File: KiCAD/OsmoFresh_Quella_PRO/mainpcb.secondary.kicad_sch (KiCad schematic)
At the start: 92 parts, among them K2 5A 250Vac, Q2 NMOS, Q3 NPN, Q4 PMOS, Q5 NPN, Q6 NPN, Q8 NPN, U4 ULN2003A

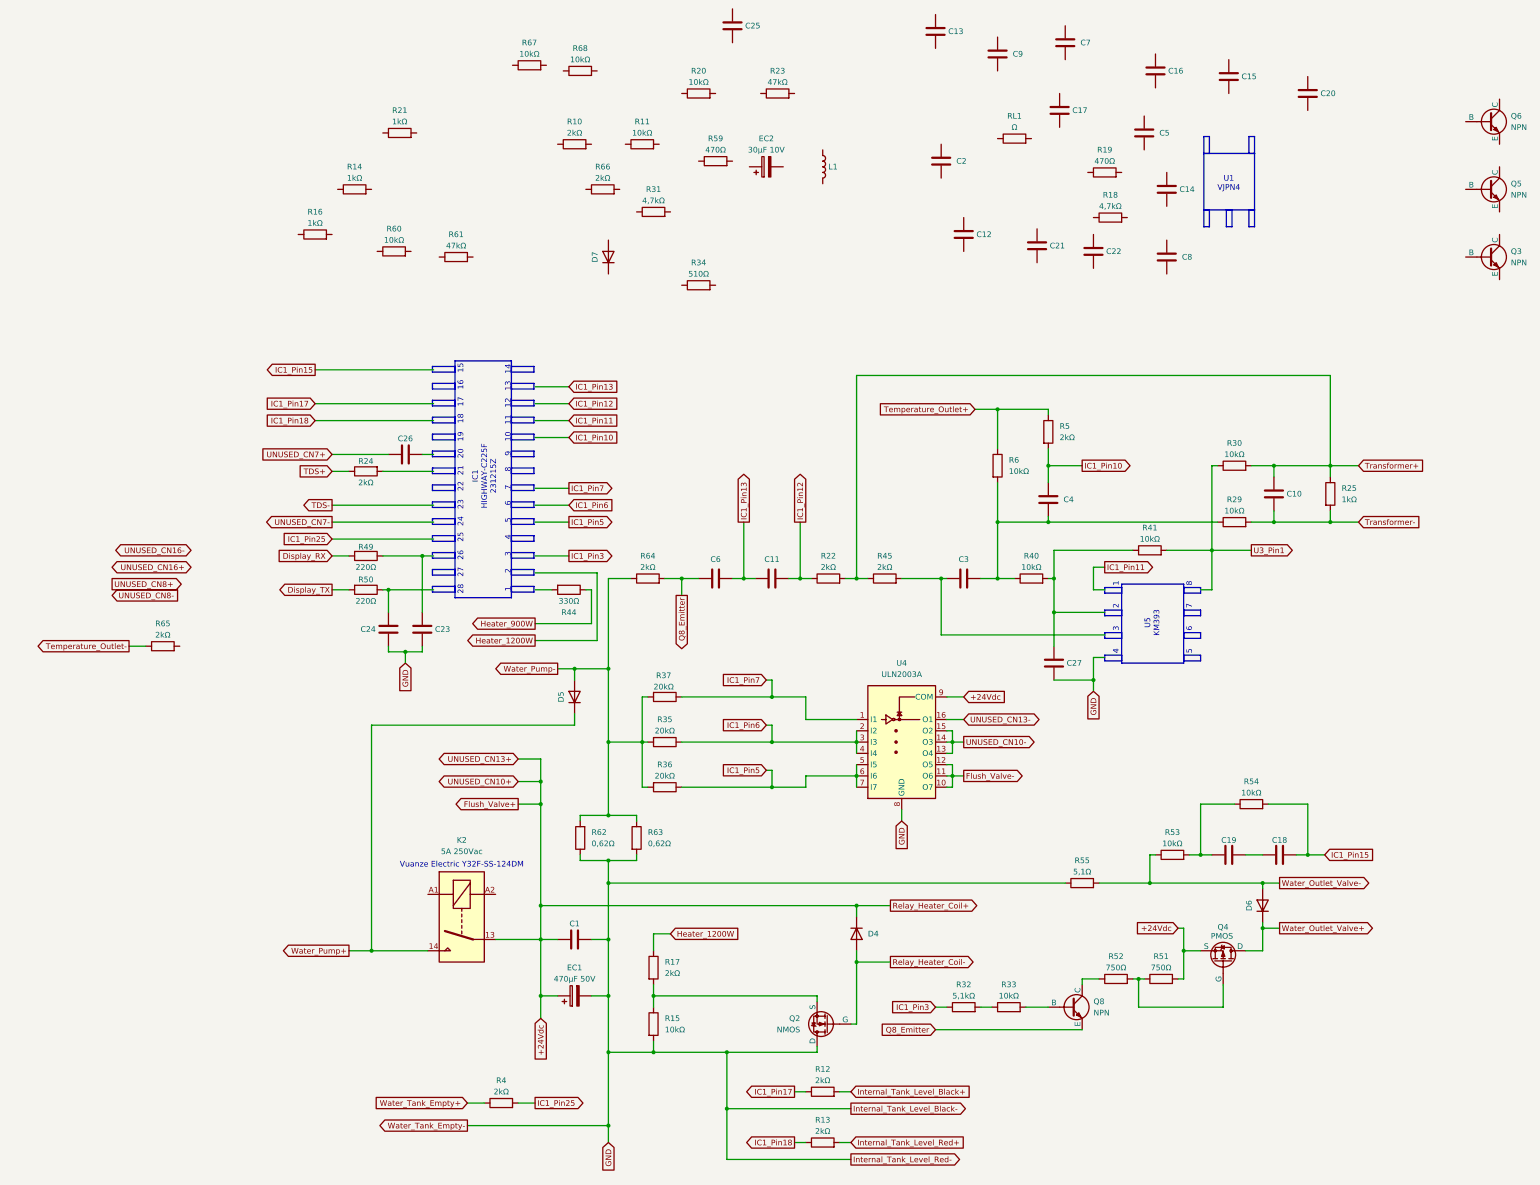
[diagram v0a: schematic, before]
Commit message: Update Schematics
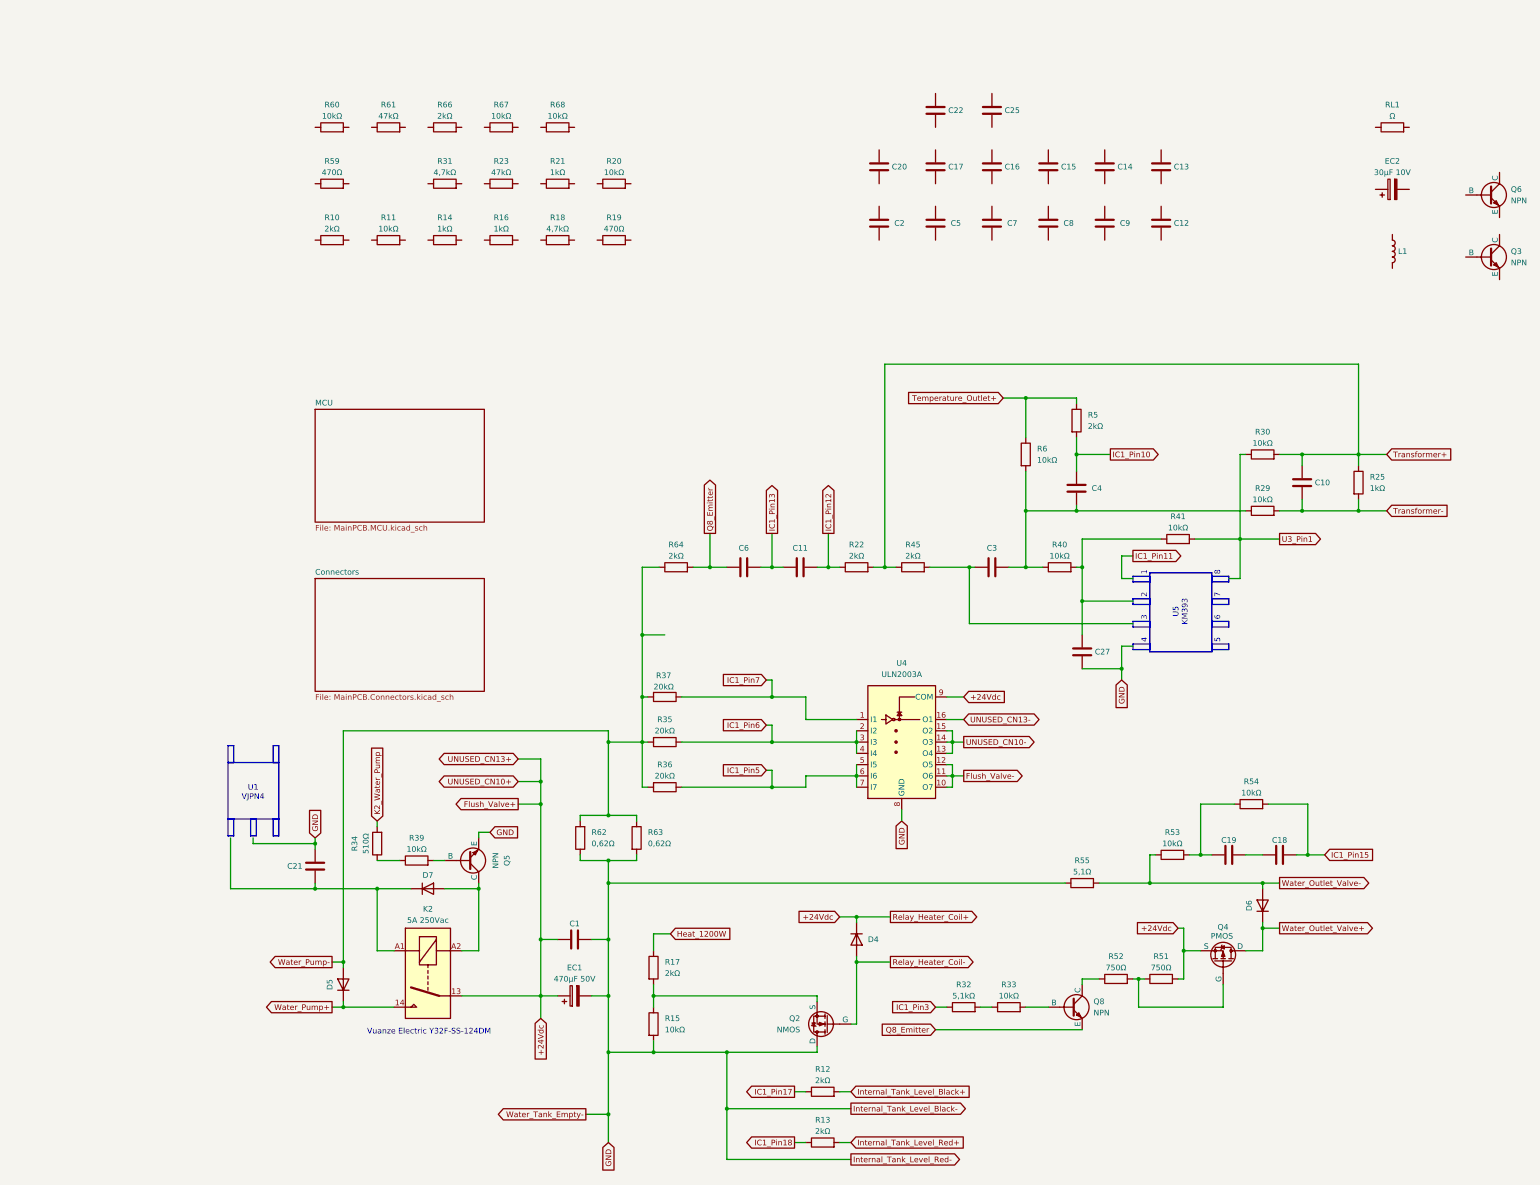
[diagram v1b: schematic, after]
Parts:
- removed C23, C24, C26: unkown, symbol Device:C
- removed D7: D, symbol Device:D
- removed R24, R4, R65: 2kΩ, symbol Device:R
- removed R44: 330Ω, symbol Device:R
- removed R49, R50: 220Ω, symbol Device:R
- added D5: D, symbol Device:D
- added R39: 10kΩ, symbol Device:R
- renumbered D5 to D7
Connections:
- net GND: now also C21.1, Q5.3 (E)
- net Water_Pump+: now also D5.1 (K); no longer D7.1 (K)
- net Water_Pump-: now also D5.2 (A); no longer D7.2 (A)
- net at Q5.1 (C): now also D7.2 (A), K2.A2
- net at Q5.2 (B): now also R39.2
- net at K2.A1: now also C21.2, D7.1 (K)
- net at R34.1: now also R39.1
- net K2_Water_Pump: now reaches R34.2
- net Heater_1200W renamed Heat_1200W
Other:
- added sheet Connectors (MainPCB.Connectors.kicad_sch)
- added sheet MCU (MainPCB.MCU.kicad_sch)
- note removed: "10"
- note removed: "11"
- note removed: "12"
- note removed: "13"
- note removed: "14"
- note removed: "15"
- note removed: "16"
- note removed: "17"
- note removed: "18"
- note removed: "19"
- note removed: "20"
- note removed: "21"
- note removed: "22"
- note removed: "23"
- note removed: "24"
- note removed: "25"
- note removed: "26"
- note removed: "27"
- note removed: "28"
- note removed: "9"
- note removed: "IC1 HIGHWAY-C225F 231215Z"
- moved on the sheet: C10, C11, C12, C13, C14, C15, C16, C17, C2, C20, C22, C25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

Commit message: Update Schematics
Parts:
- removed C14, C17, C2: unkown, symbol Device:C
- removed R12, R13: 2kΩ, symbol Device:R
- RL1: value Ω -> (none)
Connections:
- net GND: now also C11.2, C22.1, C3.2, C4.1, C6.1, Q8.3 (E), R29.1, R40.2, R6.2
- net Heat_1200W: now also R17.2; no longer R17.1
- net IC1_Pin12: now also C11.1, R22.2; no longer C11.2, R22.1
- net K2_Water_Pump: now also R34.1; no longer R34.2
- net U3_Pin1: now also R30.2; no longer R30.1
- net Water_Pump-: no longer R36.2, R64.1
- net at C27.2, R41.1: now also R40.1; no longer R40.2
- net at Q2.3 (S), R15.1: now also R17.1; no longer R17.2
- net at R39.1: now also R34.2; no longer R34.1
- net +5Vdc: now reaches RL1.1
- net +5Vdc: now also C22.2, EC2.1, L1.2
- net IC1_Pin13 renamed IC1_Pin16
- net IC1_Pin16: now also R64.2; no longer C11.1
- removed net Q8_Emitter: C6.1, Q8.3 (E), R64.2
- removed net Transformer+: C10.2, R22.2, R25.1, R30.2, R45.1
- net Transformer- renamed AC_Sense+
- net AC_Sense+: no longer R29.2
- new net: R22.1, R45.1
- new net: R36.2, R64.1
- new net AC_Sense-: C10.2, R25.1, R29.2, R30.1
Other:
- moved on the sheet: C12, C13, C15, C16, C20, C21, C25, C5, C7, C8, C9, D5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
